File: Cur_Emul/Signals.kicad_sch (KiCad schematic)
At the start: 148 parts, among them J20 Conn_01x04_Pin, J23 Conn_01x06_Pin, J24 Conn_01x08_Pin, J25 Conn_01x08_Pin, U1 Opamp_Quad, U2 Opamp_Quad, U3 Opamp_Quad, U4 Opamp_Quad, U5 MCP4922-ESL, U6 MCP4922-ESL

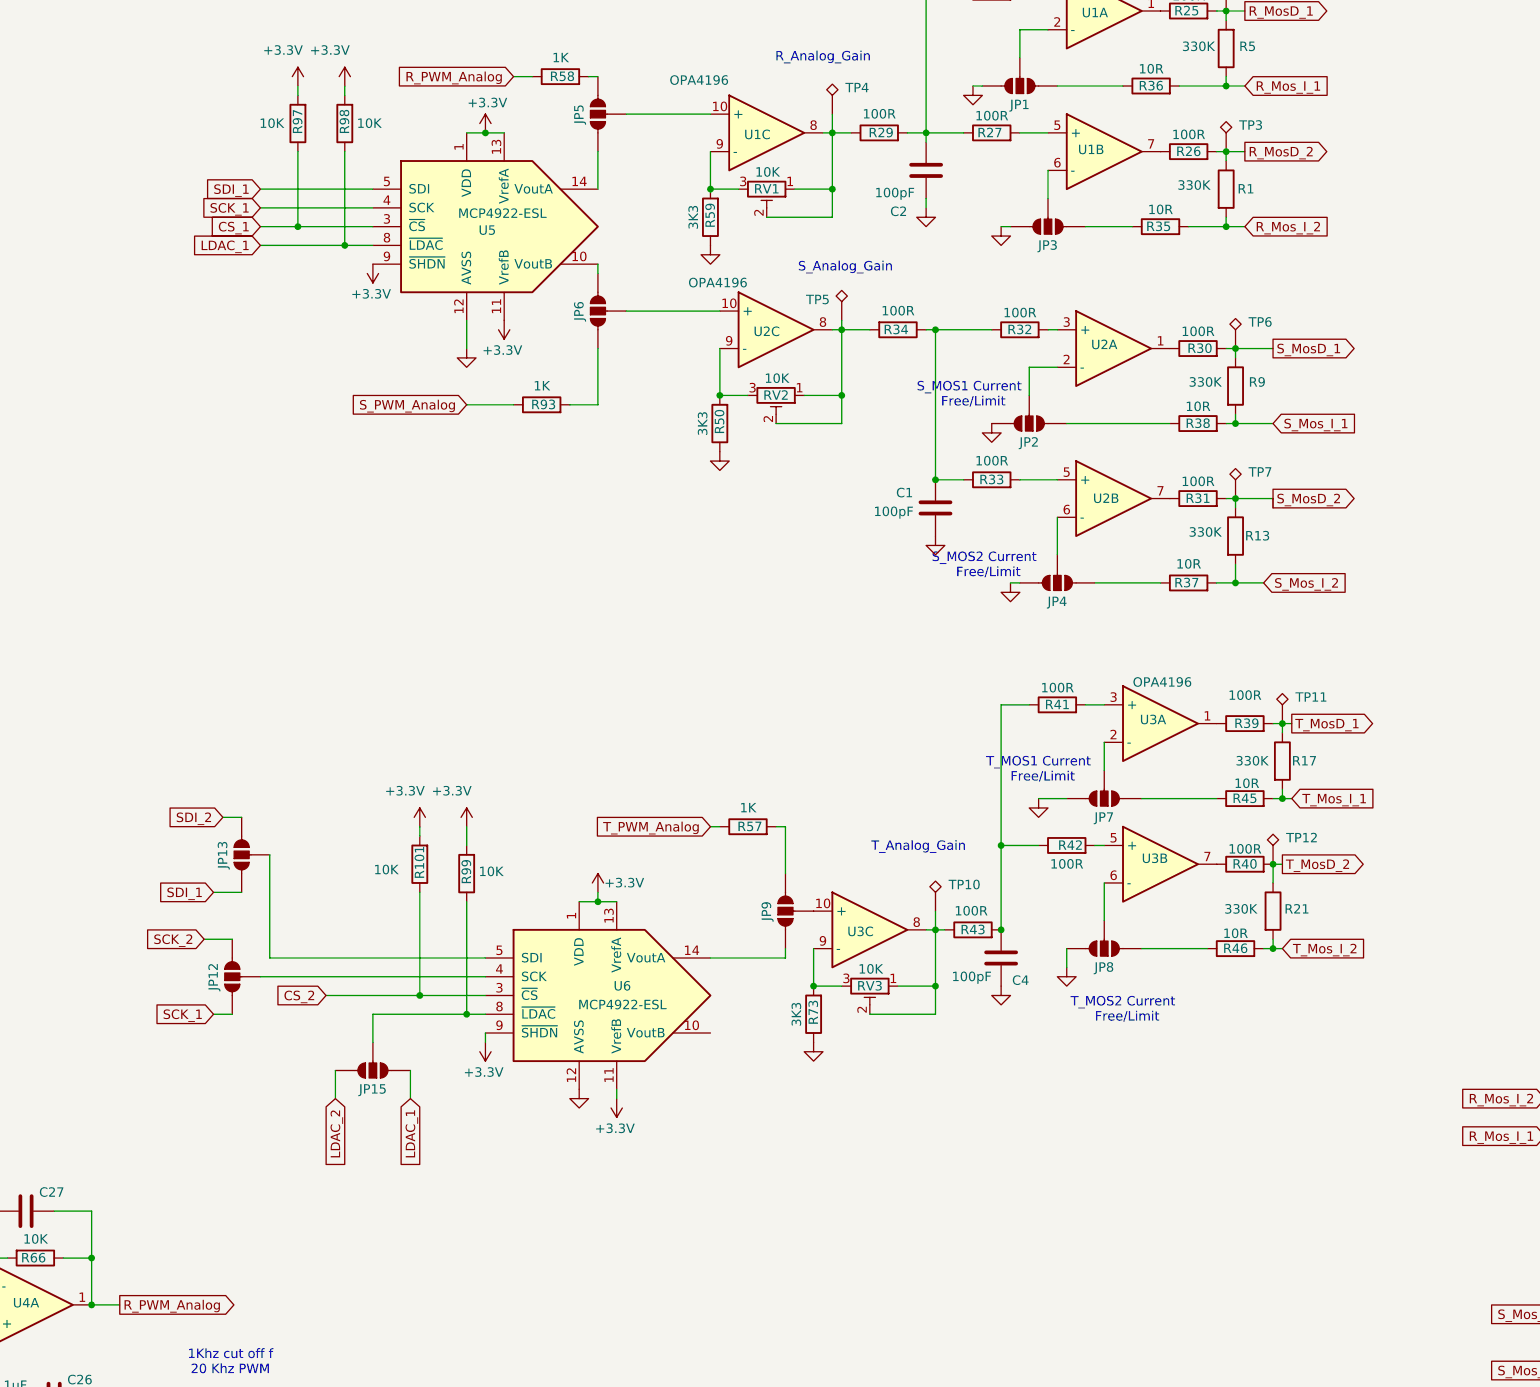
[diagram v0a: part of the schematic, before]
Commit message: updates4
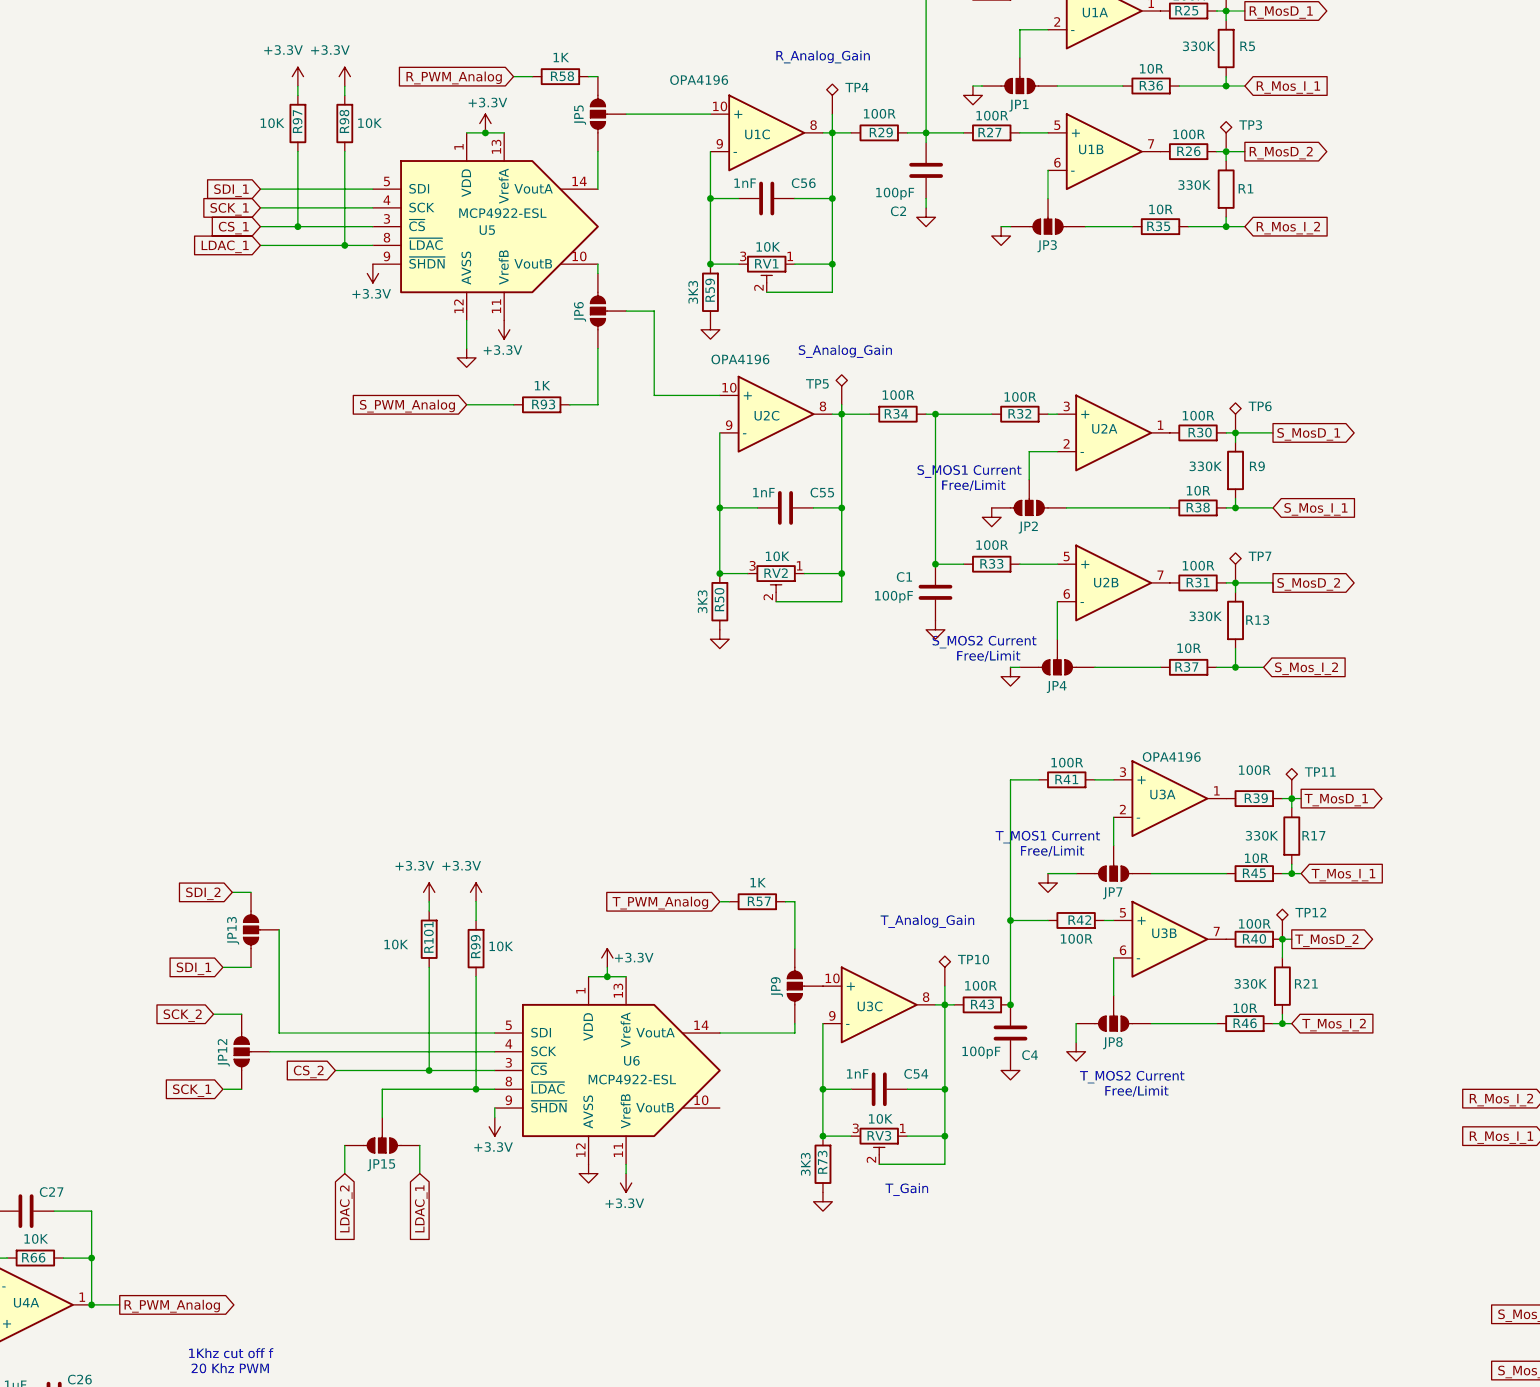
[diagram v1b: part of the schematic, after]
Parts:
- added C54, C55, C56: 1nF, Capacitor_SMD:C_0805_2012Metric_Pad1.18x1.45mm_HandSolder, symbol Device:C
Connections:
- net at R43.1, RV3.1, RV3.2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: now also C54.2
- net at R73.2, RV3.3, U3.9 (-): now also C54.1
- net at R34.2, RV2.1, RV2.2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: now also C55.2
- net at R59.2, RV1.3, U1.9 (-): now also C56.1
- net at R50.2, RV2.3, U2.9 (-): now also C55.1
- net at R29.1, RV1.1, RV1.2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: now also C56.2
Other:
- note added: "T_Gain"
- moved on the sheet: C1, C4, JP12, JP13, JP15, JP2, JP4, JP7, JP8, JP9, R101, R13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
